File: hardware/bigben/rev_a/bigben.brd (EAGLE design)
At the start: 25.6 x 13 mm, 13 parts, among them J3 IMPULSE_GECKO_HEADER, U1 RV-3049-C3, U2 FM25LBTDFN-8

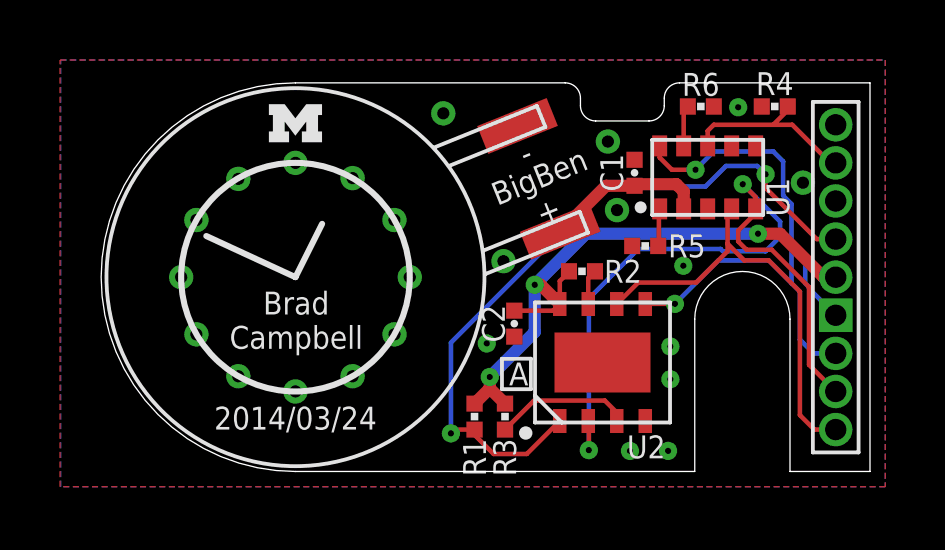
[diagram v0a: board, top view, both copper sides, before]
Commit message: bigben documentation
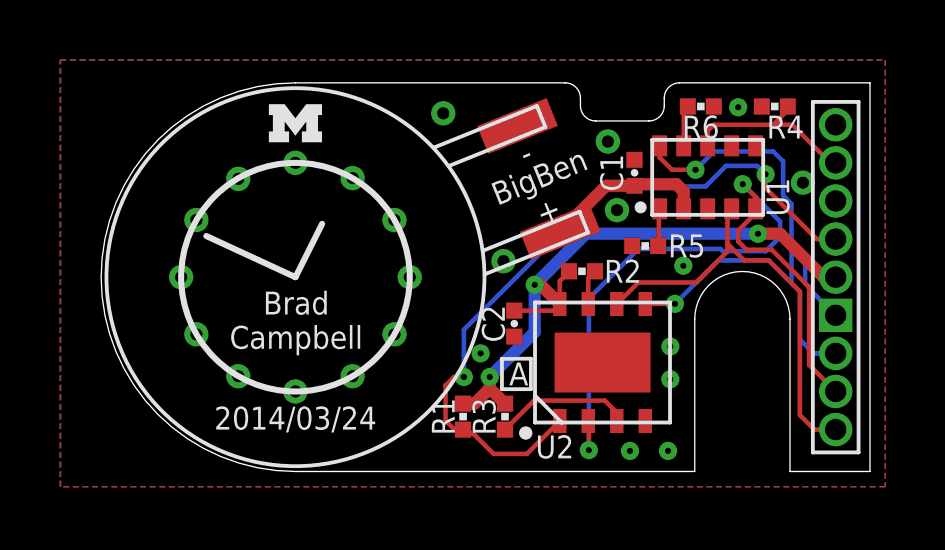
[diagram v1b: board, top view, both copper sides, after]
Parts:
- moved R1 0.38 mm to (18.9, 1.83)
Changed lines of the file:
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@@
 <element name="U2" library="chips" package="TDFN-8" value="FM25LBTDFN-8" x="23.5962" y="3.6322" smashed="yes">
 <attribute name="MOUSER" value="877-FM25V20-DG" x="23.5962" y="3.6322" size="1.778" layer="27" display="off"/>
-<attribute name="NAME" x="25.0522" y="1.201" size="0.762" layer="25" font="vector" ratio="12" rot="R180" align="bottom-center"/>
+<attribute name="NAME" x="22.0042" y="1.201" size="0.762" layer="25" font="vector" ratio="12" rot="R180" align="bottom-center"/>
 <attribute name="VALUE" x="23.5962" y="0.2322" size="0.508" layer="27" font="vector" ratio="12" align="bottom-center"/>
 </element>
-<element name="R1" library="passives" package="0402_RES" value="4.7k" x="19.3294" y="1.8288" smashed="yes" rot="R90">
-<attribute name="NAME" x="19.3294" y="1.0922" size="0.762" layer="25" font="vector" ratio="12" rot="R90" align="center-right"/>
-<attribute name="VALUE" x="19.7104" y="0.3048" size="0.508" layer="27" font="vector" ratio="12" rot="R90" align="bottom-center"/>
+<element name="R1" library="passives" package="0402_RES" value="4.7k" x="18.9484" y="1.8288" smashed="yes" rot="R90">
+<attribute name="NAME" x="18.669" y="1.8288" size="0.762" layer="25" font="vector" ratio="12" rot="R90" align="bottom-center"/>
+<attribute name="VALUE" x="19.3294" y="0.3048" size="0.508" layer="27" font="vector" ratio="12" rot="R90" align="bottom-center"/>
 </element>
 <element name="R2" library="passives" package="0402_RES" value="4.7k" x="22.9112" y="6.6728" smashed="yes" rot="R180">
@@
 </element>
 <element name="R3" library="passives" package="0402_RES" value="4.7k" x="20.3454" y="1.8288" smashed="yes" rot="R90">
-<attribute name="NAME" x="20.3348" y="1.093" size="0.762" layer="25" font="vector" ratio="12" rot="R270" align="center-left"/>
+<attribute name="NAME" x="20.03" y="1.8296" size="0.762" layer="25" font="vector" ratio="12" rot="R270" align="top-center"/>
 <attribute name="VALUE" x="21.7424" y="1.8288" size="0.508" layer="27" font="vector" ratio="12" rot="R90" align="bottom-center"/>
 </element>
@@
 </element>
 <element name="R6" library="passives" package="0402_RES" value="10k" x="26.8732" y="12.1666" smashed="yes" rot="R180">
-<attribute name="NAME" x="26.8732" y="12.5222" size="0.762" layer="25" font="vector" ratio="12" align="bottom-center"/>
+<attribute name="NAME" x="26.8732" y="11.8618" size="0.762" layer="25" font="vector" ratio="12" rot="R180" align="bottom-center"/>
 <attribute name="VALUE" x="26.8732" y="13.5636" size="1.016" layer="27" font="vector" ratio="12" rot="R180" align="bottom-center"/>
 </element>
@@
 </element>
 <element name="R4" library="passives" package="0402_RES" value="4.7k" x="29.337" y="12.1666" smashed="yes">
-<attribute name="NAME" x="29.337" y="12.5476" size="0.762" layer="25" font="vector" ratio="12" align="bottom-center"/>
+<attribute name="NAME" x="29.6926" y="11.8618" size="0.762" layer="25" font="vector" ratio="12" rot="R180" align="bottom-center"/>
 <attribute name="VALUE" x="29.337" y="10.7696" size="1.016" layer="27" font="vector" ratio="12" align="bottom-center"/>
 </element>
@@
 <via x="25.8572" y="4.1656" extent="1-16" drill="0.2032"/>
 <via x="25.8572" y="3.0734" extent="1-16" drill="0.2032"/>
-<via x="19.7358" y="4.2672" extent="1-16" drill="0.2032"/>
+<via x="19.5326" y="3.937" extent="1-16" drill="0.2032"/>
 <via x="20.2946" y="7.0104" extent="1-16" drill="0.4064"/>
 <via x="23.7744" y="10.9982" extent="1-16" drill="0.4064"/>
@@
 <wire x1="21.336" y1="4.6482" x2="19.8374" y2="3.1496" width="0.4064" layer="16"/>
 <wire x1="19.8374" y1="2.76986875" x2="20.3454" y2="2.26186875" width="0.4064" layer="1"/>
-<wire x1="19.3294" y1="2.26186875" x2="19.8374" y2="2.76986875" width="0.4064" layer="1"/>
 <wire x1="19.8374" y1="2.76986875" x2="19.8374" y2="3.1496" width="0.4064" layer="1"/>
 <wire x1="31.369" y1="6.477" x2="30.9626" y2="6.477" width="0.4064" layer="1"/>
@@
 <wire x1="29.5148" y1="7.9248" x2="28.7782" y2="7.9248" width="0.4064" layer="1"/>
 <wire x1="28.7782" y1="7.9248" x2="23.0378" y2="7.9248" width="0.4064" layer="16"/>
+<wire x1="19.8374" y1="2.76986875" x2="19.3294" y2="2.26186875" width="0.4064" layer="1"/>
+<wire x1="19.3294" y1="2.26186875" x2="18.9484" y2="2.26186875" width="0.4064" layer="1"/>
 </signal>
 <signal name="N$2">
@@
 <contactref element="J3" pad="2"/>
 <via x="29.0322" y="9.906" extent="1-16" drill="0.2032"/>
-<wire x1="23.749" y1="9.4996" x2="18.542" y2="4.2926" width="0.1524" layer="16"/>
-<wire x1="19.3294" y1="1.39573125" x2="19.3294" y2="1.2192" width="0.1524" layer="1"/>
+<wire x1="18.9484" y1="1.39573125" x2="19.3294" y2="1.2192" width="0.1524" layer="1"/>
 <wire x1="19.3294" y1="1.2192" x2="19.9644" y2="0.5842" width="0.1524" layer="1"/>
 <wire x1="19.9644" y1="0.5842" x2="21.0732" y2="0.5842" width="0.1524" layer="1"/>
 <wire x1="21.0732" y1="0.5842" x2="22.1712" y2="1.6822" width="0.1524" layer="1"/>
-<wire x1="18.542" y1="4.2926" x2="18.542" y2="1.27" width="0.1524" layer="16"/>
-<via x="18.542" y="1.27" extent="1-16" drill="0.2032"/>
-<wire x1="18.542" y1="1.27" x2="18.66773125" y2="1.39573125" width="0.1524" layer="1"/>
-<wire x1="18.66773125" y1="1.39573125" x2="19.3294" y2="1.39573125" width="0.1524" layer="1"/>
+<via x="18.9738" y="3.1496" extent="1-16" drill="0.2032"/>
+<wire x1="18.66773125" y1="1.39573125" x2="18.9484" y2="1.39573125" width="0.1524" layer="1"/>
 <wire x1="27.7114" y1="10.1854" x2="27.0256" y2="9.4996" width="0.1524" layer="16"/>
 <wire x1="27.0256" y1="9.4996" x2="23.749" y2="9.4996" width="0.1524" layer="16"/>
@@
 <wire x1="27.7114" y1="10.1854" x2="28.7528" y2="10.1854" width="0.1524" layer="16"/>
 <wire x1="28.7528" y1="10.1854" x2="29.0322" y2="9.906" width="0.1524" layer="16"/>
+<wire x1="18.66773125" y1="1.39573125" x2="18.3642" y2="1.6992625" width="0.1524" layer="1"/>
+<wire x1="18.3642" y1="1.6992625" x2="18.3642" y2="2.8702" width="0.1524" layer="1"/>
+<wire x1="18.3642" y1="2.8702" x2="18.6436" y2="3.1496" width="0.1524" layer="1"/>
+<wire x1="18.6436" y1="3.1496" x2="18.9738" y2="3.1496" width="0.1524" layer="1"/>
+<wire x1="23.749" y1="9.4996" x2="18.9738" y2="4.7244" width="0.1524" layer="16"/>
+<wire x1="18.9738" y1="4.7244" x2="18.9738" y2="3.1496" width="0.1524" layer="16"/>
 </signal>
 <signal name="!FRAM_HOLD">
